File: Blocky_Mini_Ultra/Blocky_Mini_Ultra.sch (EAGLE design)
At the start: 41 parts, among them IC3 MCP1703CB, J1 2P-2.0-90D-SMD, J2 10118193-0001LF, U1 MCP73831, X1 16 MHz, X4 12MHz

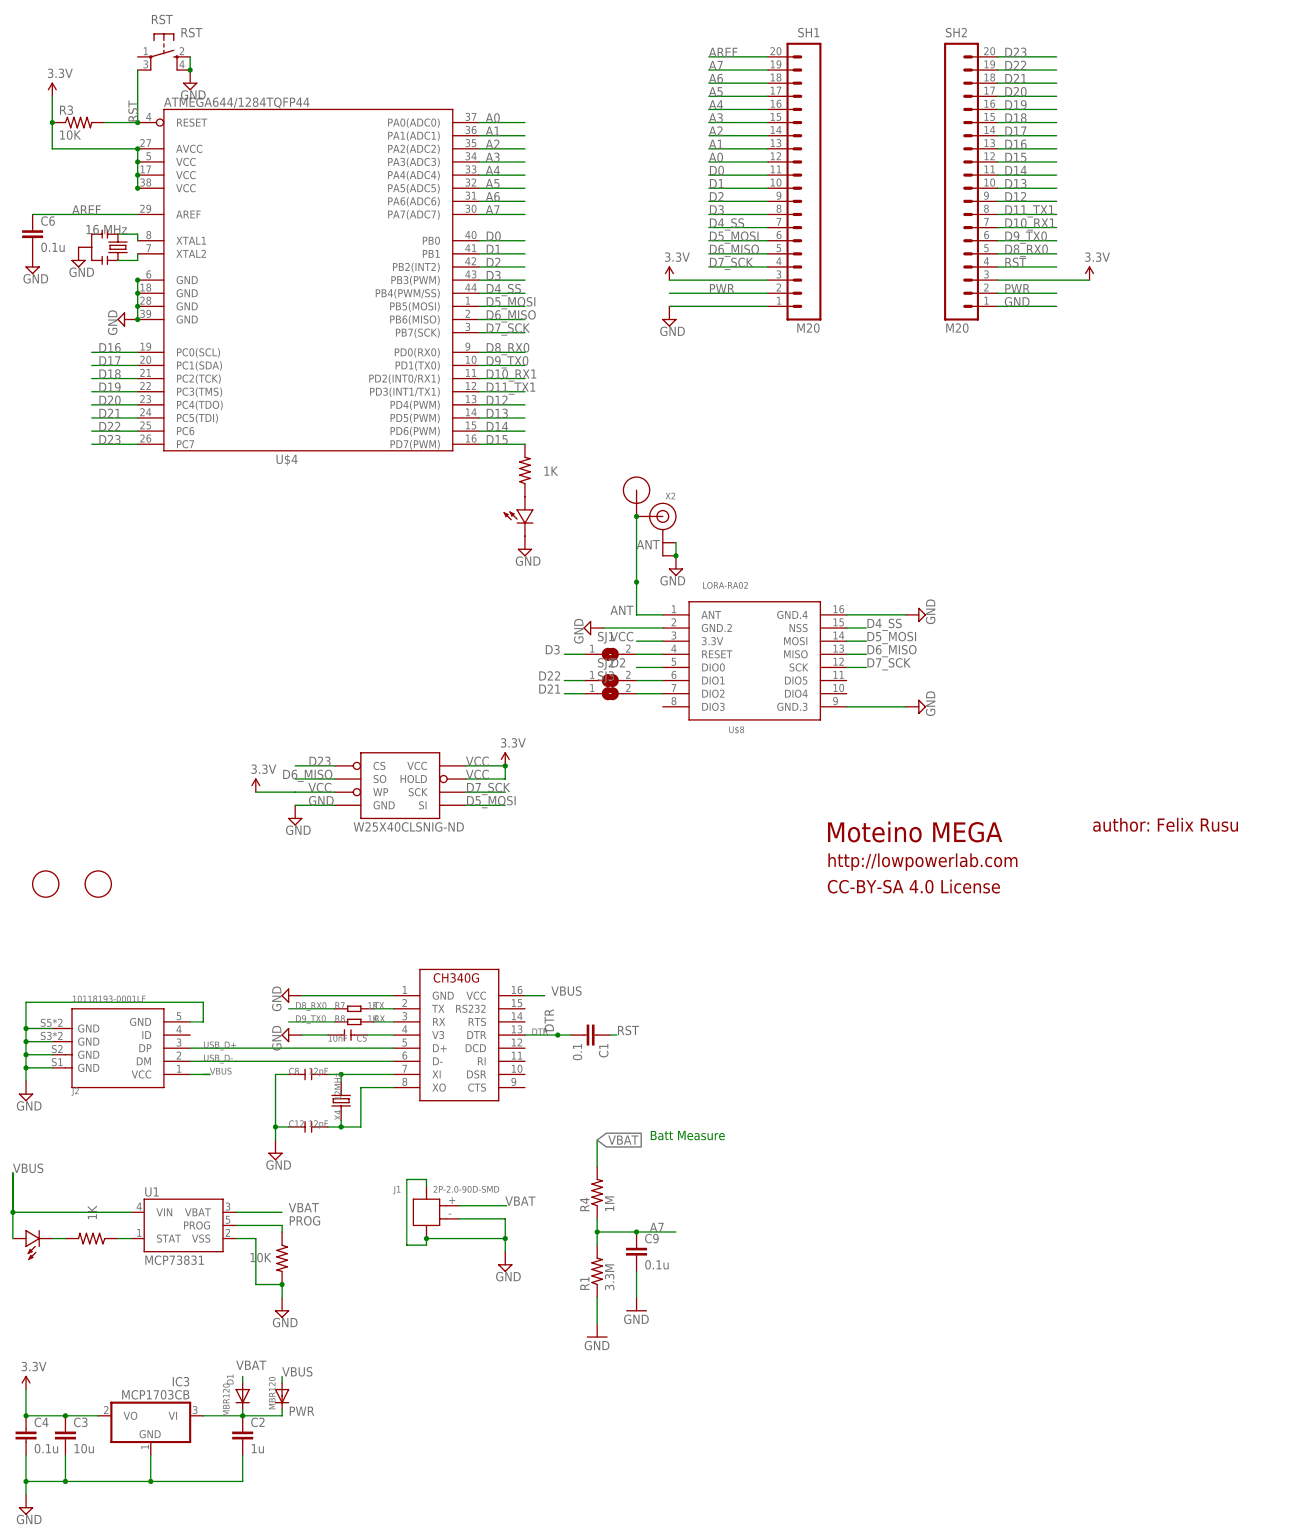
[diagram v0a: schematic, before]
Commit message: Update schematic
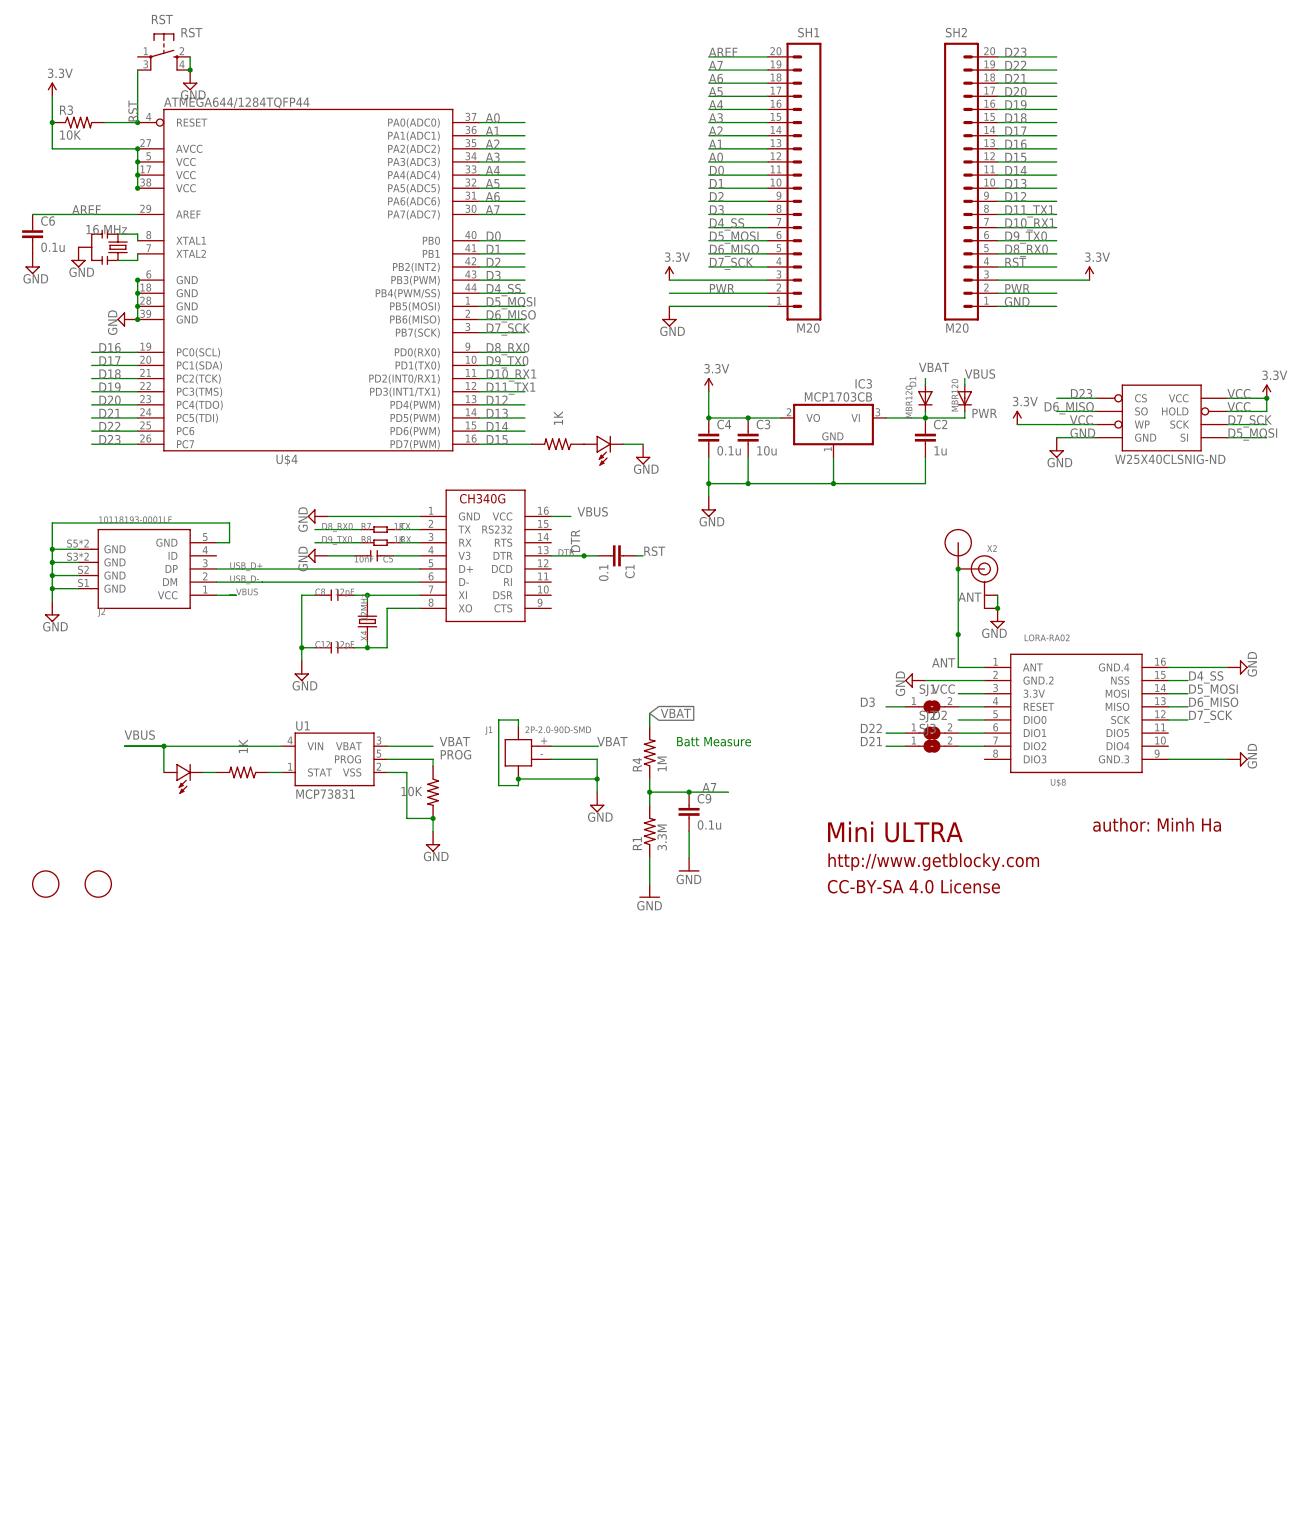
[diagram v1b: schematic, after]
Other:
- note added: "Mini ULTRA"
- note added: "author: Minh Ha"
- note added: "http://www.getblocky.com"
- note removed: "Moteino MEGA"
- note removed: "author: Felix Rusu"
- note removed: "http://lowpowerlab.com"
- moved on the sheet: C1, C12, C2, C3, C4, C5, C8, C9, D1, IC3, J1, J2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
